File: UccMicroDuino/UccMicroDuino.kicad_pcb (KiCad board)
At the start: 2 copper layers, 8 parts, among them J1 Conn_01x10_Socket, J2 USB_A, U1 ATtiny85-20S

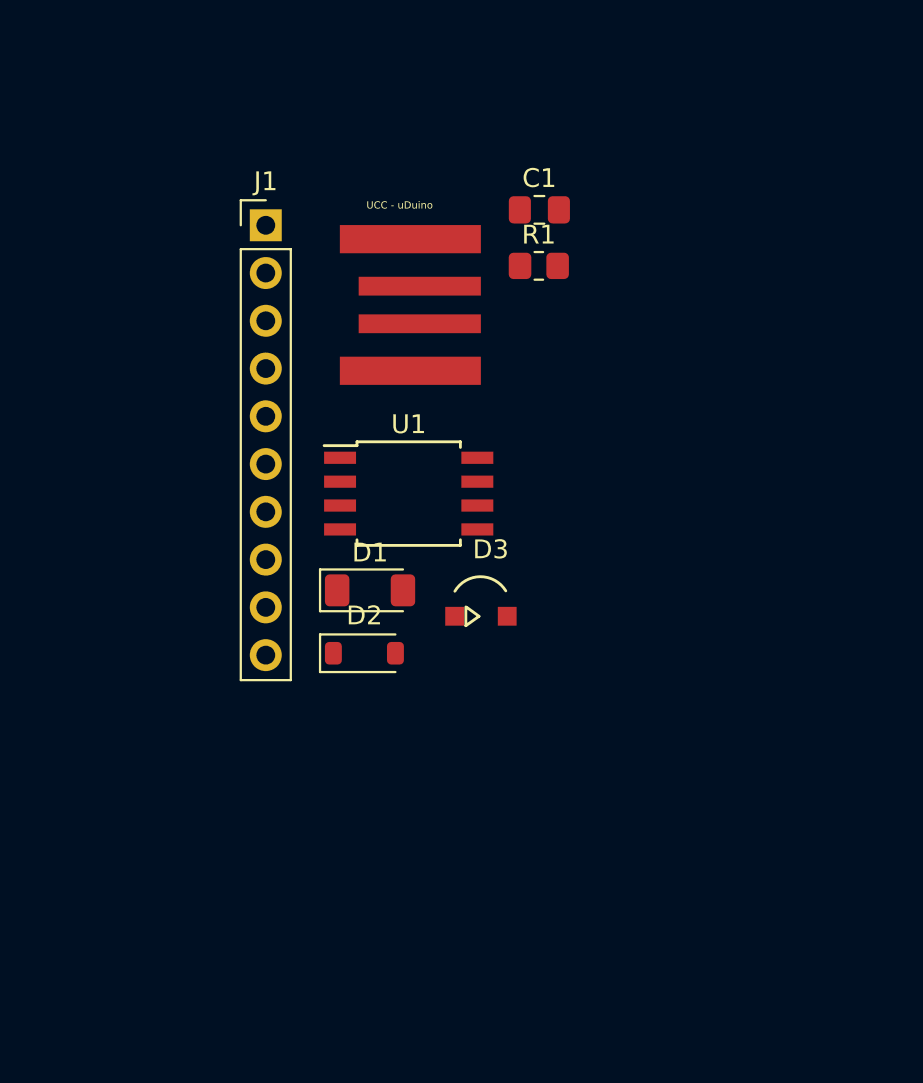
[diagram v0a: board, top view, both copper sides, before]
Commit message: Agrego proyecto UccMicroDuino
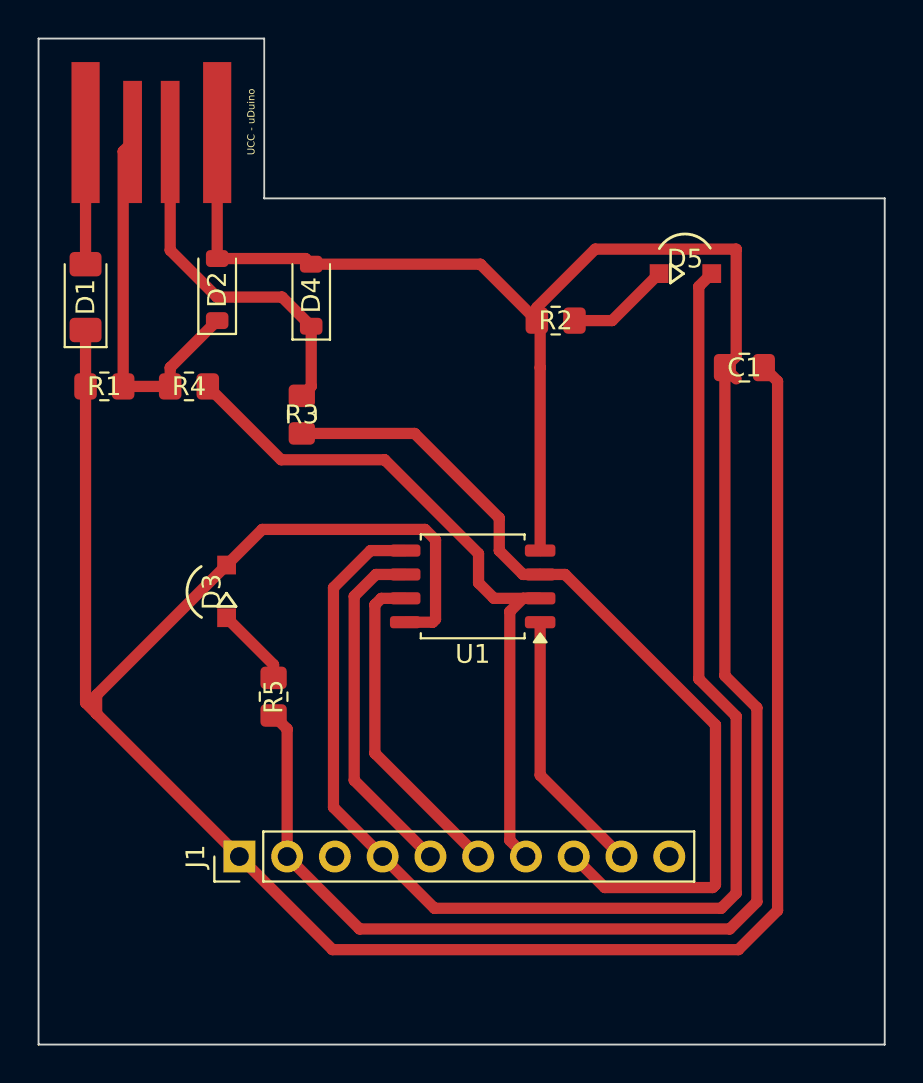
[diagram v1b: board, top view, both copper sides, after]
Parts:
- added D4: 3.6V 1/2mW, Diode_SMD:D_SOD-123, F.Cu at (126.5, 71.7)
- added D5: Led Green, ledSmd:ledSMD, F.Cu at (146.8, 70.5)
- added R2: 330Ω 5% 1/8W, Resistor_SMD:R_0805_2012Metric_Pad1.20x1.40mm_HandSolder, F.Cu at (139.5, 73.0)
- added R3: 68Ω 5% 1/8W, Resistor_SMD:R_0805_2012Metric_Pad1.20x1.40mm_HandSolder, F.Cu at (126.0, 78.0)
- added R4: 68Ω 5% 1/8W, Resistor_SMD:R_0805_2012Metric_Pad1.20x1.40mm_HandSolder, F.Cu at (120.0, 76.5)
- added R5: 330Ω 5% 1/8W, Resistor_SMD:R_0805_2012Metric_Pad1.20x1.40mm_HandSolder, F.Cu at (124.5, 93.0)
- C1: value C -> 0.1u
- D1: value D_Filled -> PMLL4148L
- D2: value D_Zener -> 3.6V 1/2mW
- D3: value LED -> Led Red
- J1: value Conn_01x10_Socket -> Header
- J2: value USB_A -> USB_PCB_A
- R1: value R -> 1.5KΩ 5% 1/8W
- U1: footprint Package_SO:SOIC-8W_5.3x5.3mm_P1.27mm -> Package_SO:SOIC-8_5.3x5.3mm_P1.27mm
- moved J1 33.6 mm to (122.7, 101.5), turned to 90 degrees
- moved R1 24.0 mm to (115.5, 76.5)
- moved D1 21.7 mm to (114.5, 71.8), turned to 90 degrees
- moved D2 20.9 mm to (121.5, 71.3), turned to 90 degrees
- moved J2 16.6 mm to (118.0, 63.2), turned to -90 degrees
- moved D3 14.0 mm to (122.0, 87.0), turned to 90 degrees
- moved C1 13.8 mm to (149.5, 75.5), turned to 180 degrees
- moved U1 5.99 mm to (135.1, 87.1), turned to 180 degrees
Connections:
- C1 pad 1: unconnected-(C1-Pad1) -> +5V
- C1 pad 2: unconnected-(C1-Pad2) -> GND
- D1 pad 2: unconnected-(D1-A-Pad2) -> Net-(D1-A)
- D2 pad 1: unconnected-(D2-K-Pad1) -> Net-(D2-K)
- D2 pad 2: unconnected-(D2-A-Pad2) -> GND
- D3 pad 1: unconnected-(D3-K-Pad1) -> Net-(D3-K)
- D3 pad 2: unconnected-(D3-A-Pad2) -> +5V
- J1 pad 1: unconnected-(J1-Pin_1-Pad1) -> +5V
- J1 pad 2: unconnected-(J1-Pin_2-Pad2) -> GND
- J1 pad 4: unconnected-(J1-Pin_4-Pad4) -> Net-(D5-A)
- J1 pad 5: unconnected-(J1-Pin_5-Pad5) -> Net-(J1-Pin_5)
- J1 pad 6: unconnected-(J1-Pin_6-Pad6) -> Net-(J1-Pin_6)
- J1 pad 7: unconnected-(J1-Pin_7-Pad7) -> Net-(J1-Pin_7)
- J1 pad 8: unconnected-(J1-Pin_8-Pad8) -> Net-(J1-Pin_8)
- J1 pad 9: unconnected-(J1-Pin_9-Pad9) -> Net-(J1-Pin_9)
- J2 pad 1: unconnected-(J2-VBUS-Pad1) -> Net-(D1-A)
- J2 pad 2: unconnected-(J2-D--Pad2) -> Net-(D2-K)
- J2 pad 3: unconnected-(J2-D+-Pad3) -> Net-(D4-K)
- J2 pad 4: unconnected-(J2-GND-Pad4) -> GND
- R1 pad 2: unconnected-(R1-Pad2) -> Net-(D2-K)
- U1 pad 1: unconnected-(U1-~{RESET}/PB5-Pad1) -> Net-(J1-Pin_9)
- U1 pad 2: unconnected-(U1-XTAL1/PB3-Pad2) -> Net-(J1-Pin_7)
- U1 pad 3: unconnected-(U1-XTAL2/PB4-Pad3) -> Net-(J1-Pin_8)
- U1 pad 4: unconnected-(U1-GND-Pad4) -> GND
- U1 pad 5: unconnected-(U1-AREF/PB0-Pad5) -> Net-(D5-A)
- U1 pad 6: unconnected-(U1-PB1-Pad6) -> Net-(J1-Pin_5)
- U1 pad 7: unconnected-(U1-PB2-Pad7) -> Net-(J1-Pin_6)
- U1 pad 8: unconnected-(U1-VCC-Pad8) -> +5V
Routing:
- net GND: track 0.00 -> 121.4 mm
- net +5V: track 0.00 -> 120.9 mm
- net Net-(D5-A): track 0.00 -> 74.3 mm
- net Net-(J1-Pin_8): track 0.00 -> 46.2 mm
- net Net-(J1-Pin_7): track 0.00 -> 38.5 mm
- net Net-(D2-K): track 0.00 -> 20.2 mm
- net Net-(D4-K): track 0.00 -> 18.8 mm
- net Net-(J1-Pin_5): track 0.00 -> 18.7 mm
- net Net-(J1-Pin_6): track 0.00 -> 17.4 mm
- net Net-(J1-Pin_9): track 0.00 -> 14.3 mm
- net Net-(D1-A): track 0.00 -> 7.00 mm
- net Net-(D5-K): track 0.00 -> 5.54 mm
- net Net-(D3-K): track 0.00 -> 4.24 mm
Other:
- board outline added: 45 x 53.5 mm
